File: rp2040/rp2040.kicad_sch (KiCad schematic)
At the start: 1 part, among them U1 RP2040

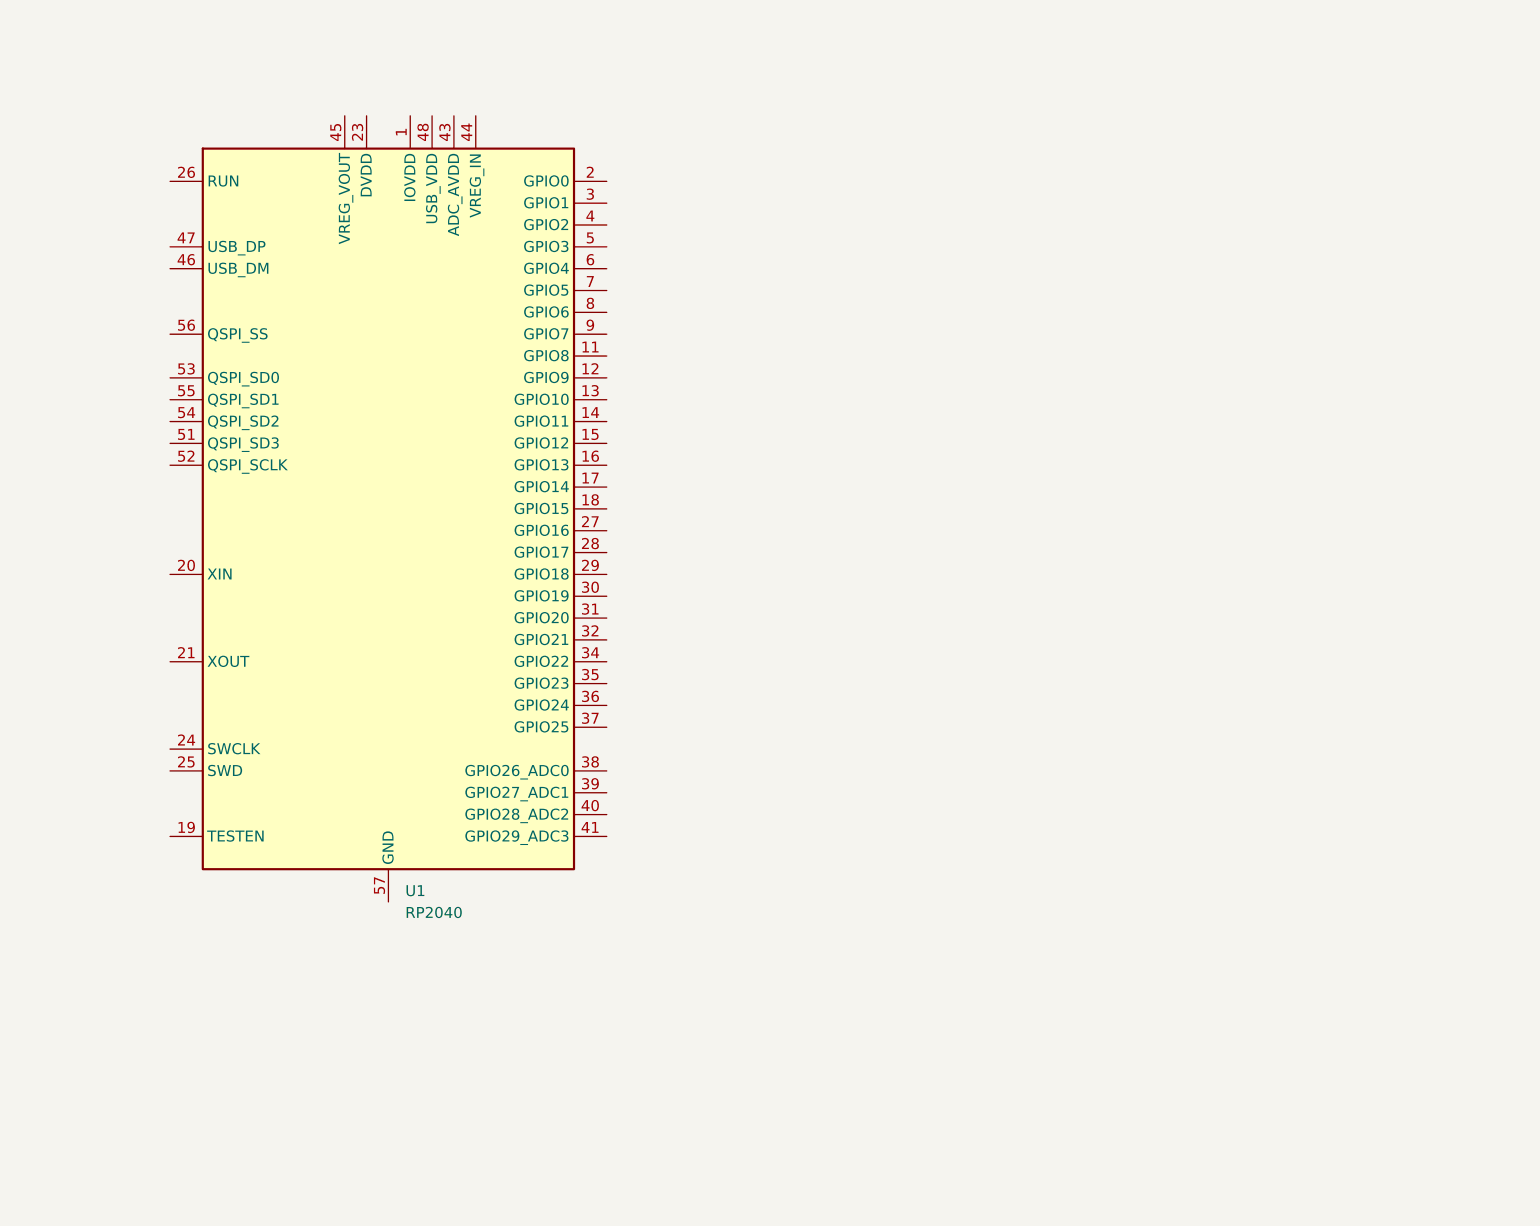
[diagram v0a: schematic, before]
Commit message: .
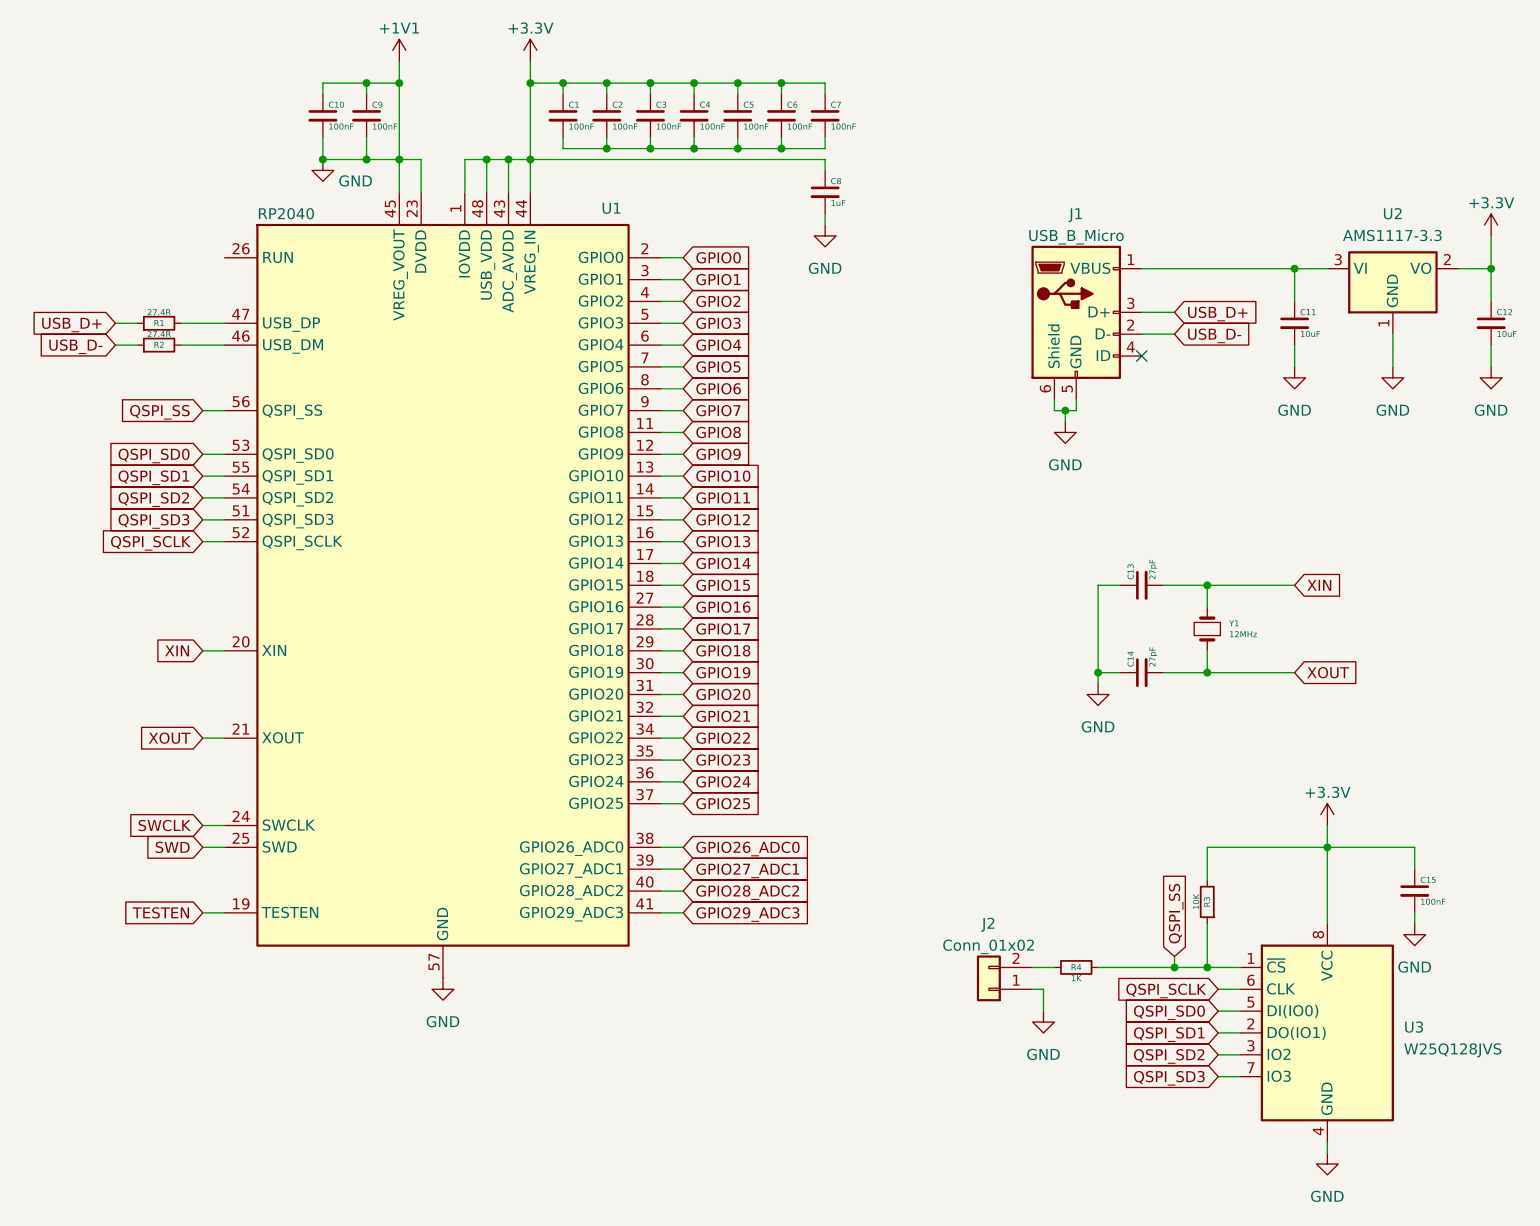
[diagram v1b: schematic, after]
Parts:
- added C1, C10, C15, C2, C3, C4, C5, C6, C7, C9: 100nF, Capacitor_SMD:C_0603_1608Metric, symbol Device:C_Small
- added C11, C12: 10uF, Capacitor_SMD:C_0603_1608Metric, symbol Device:C_Small
- added C13, C14: 27pF, Capacitor_SMD:C_0603_1608Metric, symbol Device:C_Small
- added C8: 1uF, Capacitor_SMD:C_0603_1608Metric, symbol Device:C_Small
- added J1: USB_B_Micro, Connector_USB:USB_Micro-B_GCT_USB3076-30-A, symbol Connector:USB_B_Micro
- added J2: Conn_01x02, symbol Connector_Generic:Conn_01x02
- added R1, R2: 27.4R, symbol Device:R_Small
- added R3: 10K, symbol Device:R_Small
- added R4: 1K, symbol Device:R_Small
- added U2: AMS1117-3.3, Package_TO_SOT_SMD:SOT-223-3_TabPin2, symbol Regulator_Linear:AMS1117-3.3
- added U3: W25Q128JVS, Package_SO:SOIC-8_5.23x5.23mm_P1.27mm, symbol Memory_Flash:W25Q128JVS
- added Y1: 12MHz, symbol Device:Crystal_Small
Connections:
- net +3.3V: now reaches U1.1 (IOVDD), U1.10 (IOVDD), U1.22 (IOVDD), U1.33 (IOVDD), U1.42 (IOVDD), U1.49 (IOVDD)
- net +3.3V: now also U1.43 (ADC_AVDD), U1.44 (VREG_IN), U1.48 (USB_VDD), C1.1, C12.1, C15.1, C2.1, C3.1, C4.1, C5.1, C6.1, C7.1, C8.1, R3.2, U2.2 (VO), U3.8 (VCC)
- net GPIO8: now reaches U1.11 (GPIO8)
- net GPIO9: now reaches U1.12 (GPIO9)
- net GPIO10: now reaches U1.13 (GPIO10)
- net GPIO11: now reaches U1.14 (GPIO11)
- net GPIO12: now reaches U1.15 (GPIO12)
- net GPIO13: now reaches U1.16 (GPIO13)
- net GPIO14: now reaches U1.17 (GPIO14)
- net GPIO15: now reaches U1.18 (GPIO15)
- net TESTEN: now reaches U1.19 (TESTEN)
- net GPIO0: now reaches U1.2 (GPIO0)
- net XIN: now reaches U1.20 (XIN)
- net XIN: now also C13.2, Y1.2
- net XOUT: now reaches U1.21 (XOUT)
- net XOUT: now also C14.2, Y1.1
- net +1V1: now reaches U1.23 (DVDD), U1.50 (DVDD)
- net +1V1: now also U1.45 (VREG_VOUT), U1.57 (GND), C10.1, C10.2, C11.2, C12.2, C13.1, C14.1, C15.2, C8.2, C9.1, C9.2, J1.5 (GND), J1.6 (Shield), J2.1 (Pin_1), U2.1 (GND), U3.4 (GND)
- net SWCLK: now reaches U1.24 (SWCLK)
- net SWD: now reaches U1.25 (SWD)
- net GPIO16: now reaches U1.27 (GPIO16)
- net GPIO17: now reaches U1.28 (GPIO17)
- net GPIO18: now reaches U1.29 (GPIO18)
- net GPIO1: now reaches U1.3 (GPIO1)
- net GPIO19: now reaches U1.30 (GPIO19)
- net GPIO20: now reaches U1.31 (GPIO20)
- net GPIO21: now reaches U1.32 (GPIO21)
- net GPIO22: now reaches U1.34 (GPIO22)
- net GPIO23: now reaches U1.35 (GPIO23)
- net GPIO24: now reaches U1.36 (GPIO24)
- net GPIO25: now reaches U1.37 (GPIO25)
- net GPIO26_ADC0: now reaches U1.38 (GPIO26_ADC0)
- net GPIO27_ADC1: now reaches U1.39 (GPIO27_ADC1)
- net GPIO2: now reaches U1.4 (GPIO2)
- net GPIO28_ADC2: now reaches U1.40 (GPIO28_ADC2)
- net GPIO29_ADC3: now reaches U1.41 (GPIO29_ADC3)
- net at U1.46 (USB_DM): now also R2.2
- net at U1.47 (USB_DP): now also R1.2
- net GPIO3: now reaches U1.5 (GPIO3)
- net QSPI_SD3: now reaches U1.51 (QSPI_SD3)
- net QSPI_SD3: now also U3.7 (IO3)
- net QSPI_SCLK: now reaches U1.52 (QSPI_SCLK)
- net QSPI_SCLK: now also U3.6 (CLK)
- net QSPI_SD0: now reaches U1.53 (QSPI_SD0)
- net QSPI_SD0: now also U3.5 (DI(IO0))
- net QSPI_SD2: now reaches U1.54 (QSPI_SD2)
- net QSPI_SD2: now also U3.3 (IO2)
- net QSPI_SD1: now reaches U1.55 (QSPI_SD1)
- net QSPI_SD1: now also U3.2 (DO(IO1))
- net QSPI_SS: now reaches U1.56 (QSPI_SS)
- net QSPI_SS: now also R3.1, R4.1, U3.1 (~{CS})
- net GPIO4: now reaches U1.6 (GPIO4)
- net GPIO5: now reaches U1.7 (GPIO5)
- net GPIO6: now reaches U1.8 (GPIO6)
- net GPIO7: now reaches U1.9 (GPIO7)
- new net: C11.1, J1.1 (VBUS), U2.3 (VI)
- new net: C1.2, C2.2, C3.2, C4.2, C5.2, C6.2, C7.2
- new net: J2.2 (Pin_2), R4.2
- new net USB_D+: J1.3 (D+), R1.1
- new net USB_D-: J1.2 (D-), R2.1
- no-connect marks 0 -> 1
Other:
- moved on the sheet: U1
